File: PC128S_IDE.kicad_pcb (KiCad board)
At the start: 2 copper layers, 61.5 x 50.7 mm, 15 parts, among them J1 User 2MHZ Port, J3 Conn_01x02_Male, J5 Conn_01x02_Male, P1 IDE02x20, U1 74HCT02, U2 74HCT139

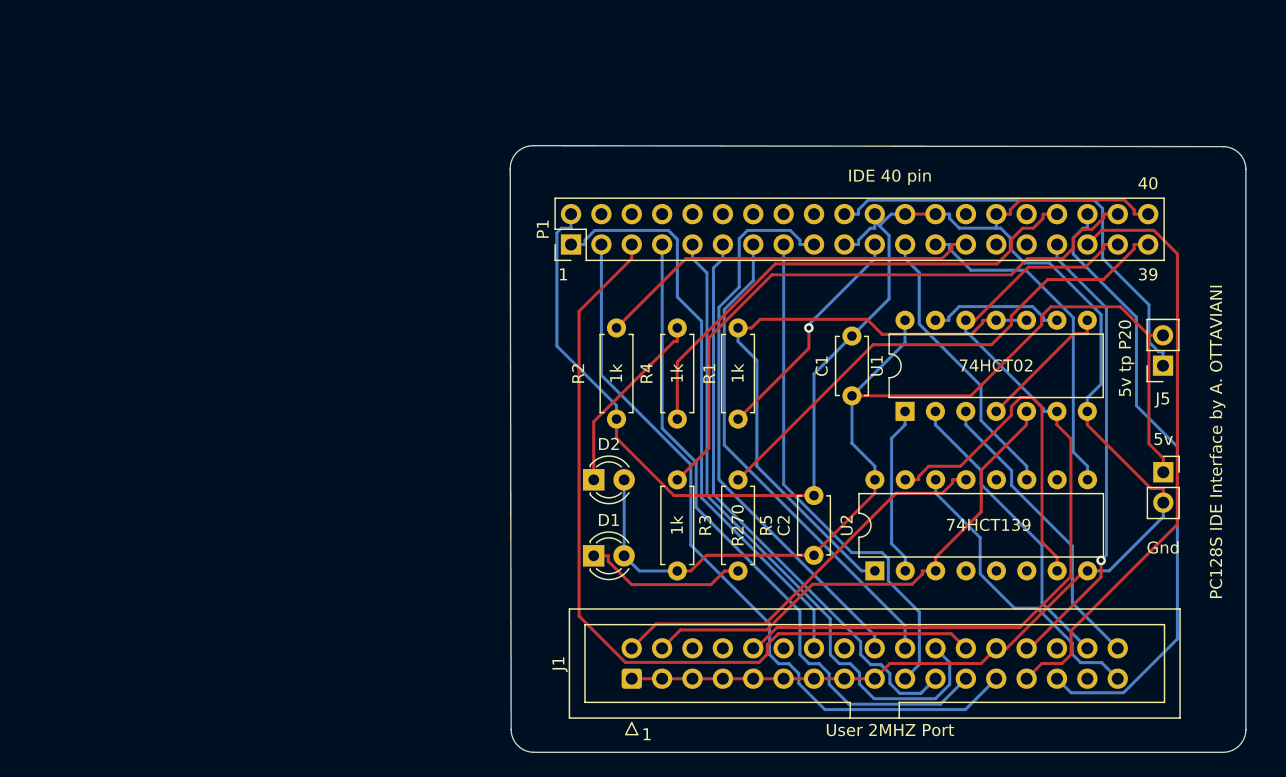
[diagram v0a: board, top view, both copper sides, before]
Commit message: Add files via upload
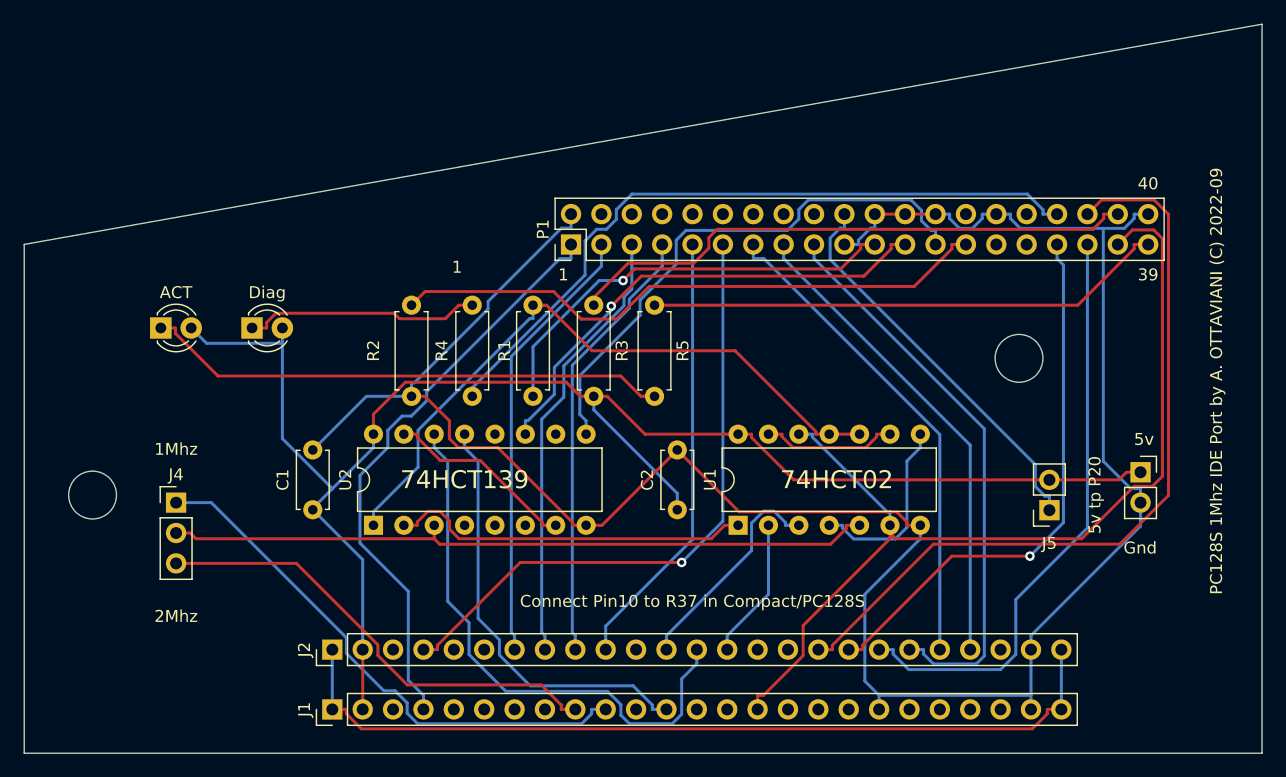
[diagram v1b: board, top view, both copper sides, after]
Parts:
- removed D1, D2: LED, LED_THT:LED_D3.0mm
- added ACT: LED, LED_THT:LED_D3.0mm, F.Cu at (130.2, 88.9)
- added Diag: LED, LED_THT:LED_D3.0mm, F.Cu at (137.8, 88.9)
- added J2: B1-25, Connector_PinHeader_2.54mm:PinHeader_1x25_P2.54mm_Vertical, F.Cu at (144.5, 115.8)
- added J4: ClockSwitch, Connector_PinHeader_2.54mm:PinHeader_1x03_P2.54mm_Vertical, F.Cu at (131.4, 103.5)
- J1: value User 2MHZ Port -> A1-25; footprint Connector_IDC:IDC-Header_2x17_P2.54mm_Vertical -> Connector_PinHeader_2.54mm:PinHeader_1x25_P2.54mm_Vertical
- moved C1 46.1 mm to (142.9, 104.1)
- moved U2 42.1 mm to (147.9, 105.4)
- moved J1 25.2 mm to (144.5, 120.8)
- moved R1 17.3 mm to (161.3, 94.6)
- moved R2 17.3 mm to (151.1, 87.0)
- moved R4 17.3 mm to (156.2, 94.6)
- moved U1 16.9 mm to (178.4, 105.4)
- moved R5 16.2 mm to (171.4, 87.0)
- moved R3 16.2 mm to (166.4, 87.0)
- moved J5 15.4 mm to (204.5, 104.1)
- moved C2 12.0 mm to (173.4, 104.1)
- moved J3 1.91 mm to (212.1, 101.0)
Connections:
- J1 pad 1: GND -> ScreenGND
- J1 pad 10: ~{INFC} -> 1MHZ
- J1 pad 11: GND -> unconnected-(J1-Pad11)
- J1 pad 12: unconnected-(J1-Pad12) -> R~{W}
- J1 pad 13: GND -> unconnected-(J1-Pad13)
- J1 pad 14: ~{RST} -> unconnected-(J1-Pad14)
- J1 pad 15: GND -> ~{INFC}
- J1 pad 17: GND -> unconnected-(J1-Pad17)
- J1 pad 18: D0 -> unconnected-(J1-Pad18)
- J1 pad 19: D1 -> GND
- J1 pad 2: R~{W} -> +5V
- J1 pad 20: D2 -> unconnected-(J1-Pad20)
- J1 pad 21: D3 -> unconnected-(J1-Pad21)
- J1 pad 22: D4 -> unconnected-(J1-Pad22)
- J1 pad 23: D5 -> unconnected-(J1-Pad23)
- J1 pad 24: D6 -> GND
- J1 pad 25: D7 -> ScreenGND
- J1 pad 3: GND -> unconnected-(J1-Pad3)
- J1 pad 4: Clock -> ~{RST}
- J1 pad 5: GND -> unconnected-(J1-Pad5)
- J1 pad 7: GND -> unconnected-(J1-Pad7)
- J1 pad 9: GND -> PHI2
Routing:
- net ScreenGND: track 0.00 -> 72.7 mm
- net 1MHZ: track 0.00 -> 45.6 mm
- net +5V: track 90.2 -> 133.3 mm
- net PHI2: track 0.00 -> 39.2 mm
- net D6: track 68.8 -> 37.1 mm
- net Net-(R5-Pad2): track 13.8 -> 43.9 mm
- net D7: track 62.5 -> 37.1 mm
- net A6: track 25.1 -> 46.6 mm
- net D5: track 56.1 -> 37.1 mm
- net IORDY: track 32.3 -> 50.6 mm
- net D4: track 55.1 -> 36.9 mm
- net ~{RD}: track 28.3 -> 46.1 mm
- net Clock: track 42.2 -> 59.5 mm
- net DMRQ: track 19.3 -> 36.5 mm
- net ~{DIAG}: track 42.4 -> 59.4 mm
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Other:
- board size 61.5 x 50.7 mm -> 103.5 x 61 mm
- board text added: "1Mhz"
- board text added: "2Mhz"
- board text added: "74HCT02"
- board text added: "74HCT139"
- board text added: "Connect Pin10 to R37 in Compact/PC128S"
- board text added: "PC128S 1Mhz IDE Port by A. OTTAVIANI (C) 2022-09"
- board text removed: "IDE 40 pin"
- board text removed: "PC128S IDE Interface by A. OTTAVIANI"

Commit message: Add files via upload
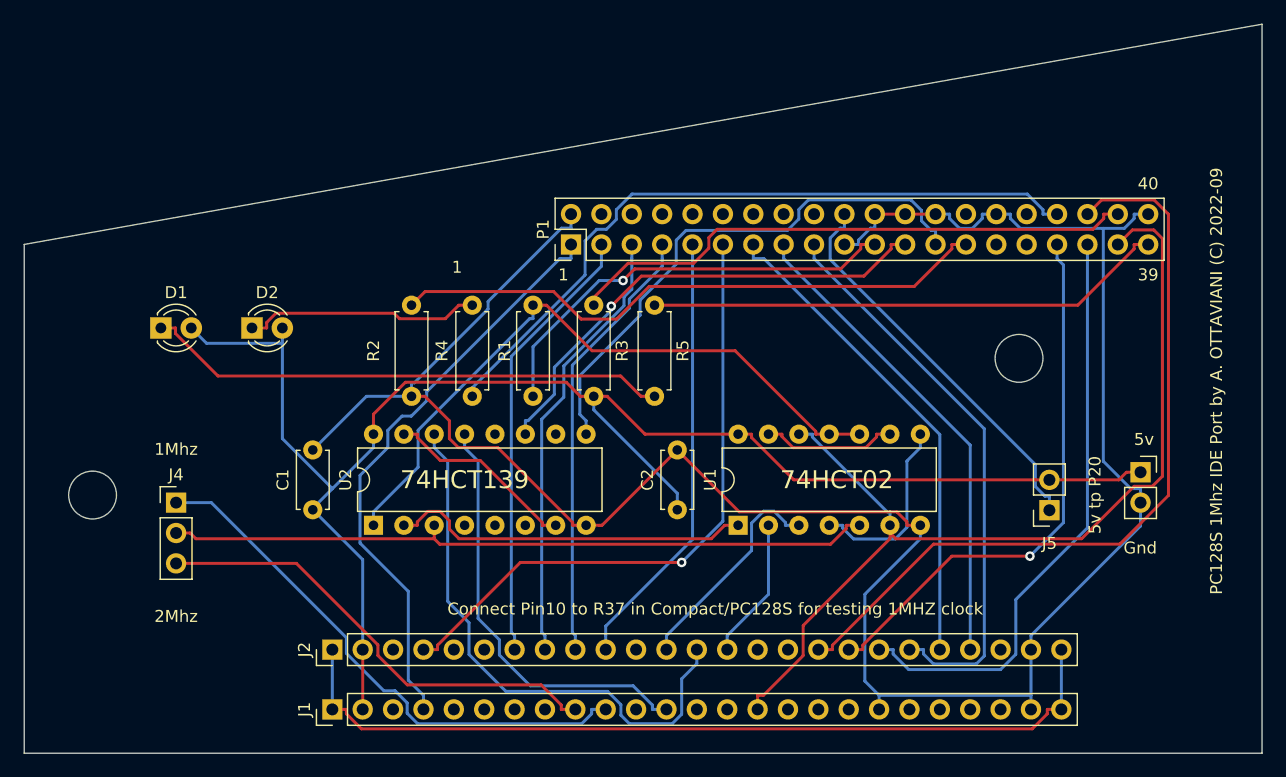
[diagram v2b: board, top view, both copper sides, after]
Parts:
- removed ACT, Diag: LED, LED_THT:LED_D3.0mm
- added D1: LED, LED_THT:LED_D3.0mm, F.Cu at (130.2, 88.9)
- added D2: LED, LED_THT:LED_D3.0mm, F.Cu at (137.8, 88.9)
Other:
- board text added: "Connect Pin10 to R37 in Compact/PC128S for testing 1MHZ clock"
- board text removed: "Connect Pin10 to R37 in Compact/PC128S"
